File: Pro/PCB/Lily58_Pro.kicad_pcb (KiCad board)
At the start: 2 copper layers, 142.5 x 111.4 mm, 58 parts, among them J1 OLED, J2 TRRS, SW1 SW_PUSH, SW10 SW_PUSH, SW11 SW_PUSH, SW12 SW_PUSH, SW13 SW_PUSH, SW14 SW_PUSH, SW15 SW_PUSH, SW16 SW_PUSH, SW17 SW_PUSH, SW18 SW_PUSH, SW19 SW_PUSH, SW2 SW_PUSH, SW20 SW_PUSH, SW21 SW_PUSH, SW22 SW_PUSH, SW23 SW_PUSH, SW24 SW_PUSH, SW25 SW_PUSH, SW26 SW_PUSH, SW27 SW_PUSH, SW28 SW_PUSH, SW29 SW_PUSH, SW3 SW_PUSH, SW4 SW_PUSH, SW5 SW_PUSH, SW6 SW_PUSH, SW7 SW_PUSH, SW8 SW_PUSH, SW9 SW_PUSH

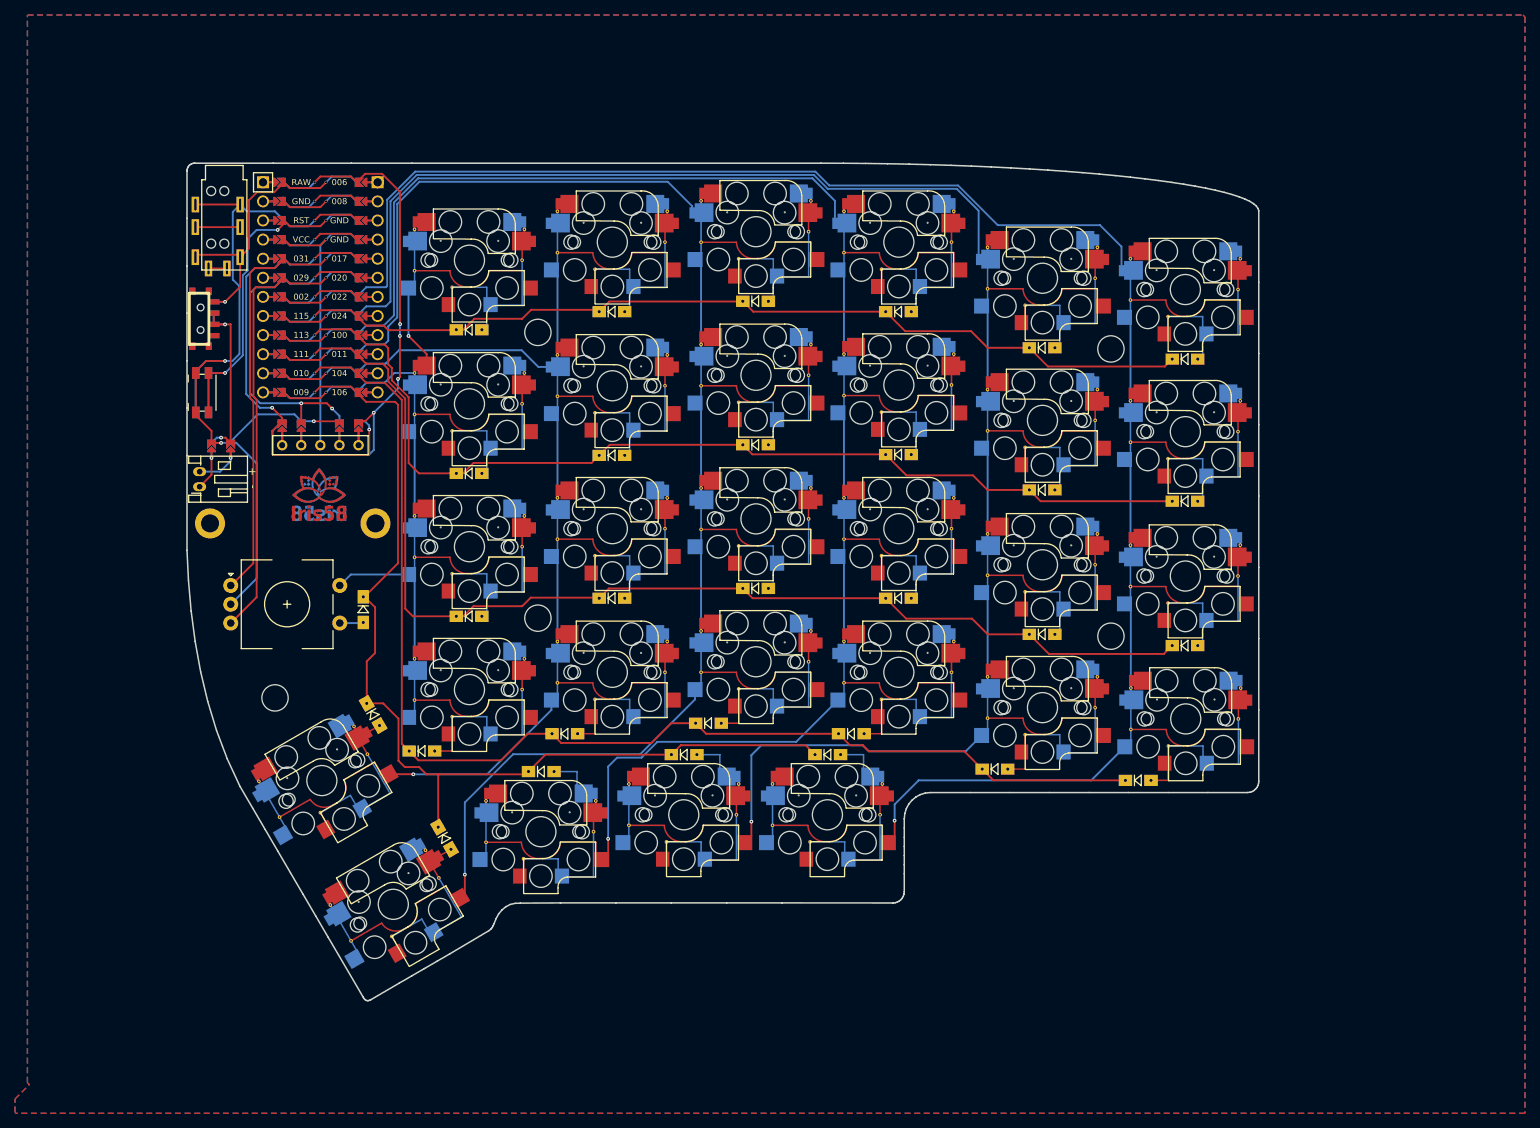
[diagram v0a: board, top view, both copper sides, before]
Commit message: Small fixes
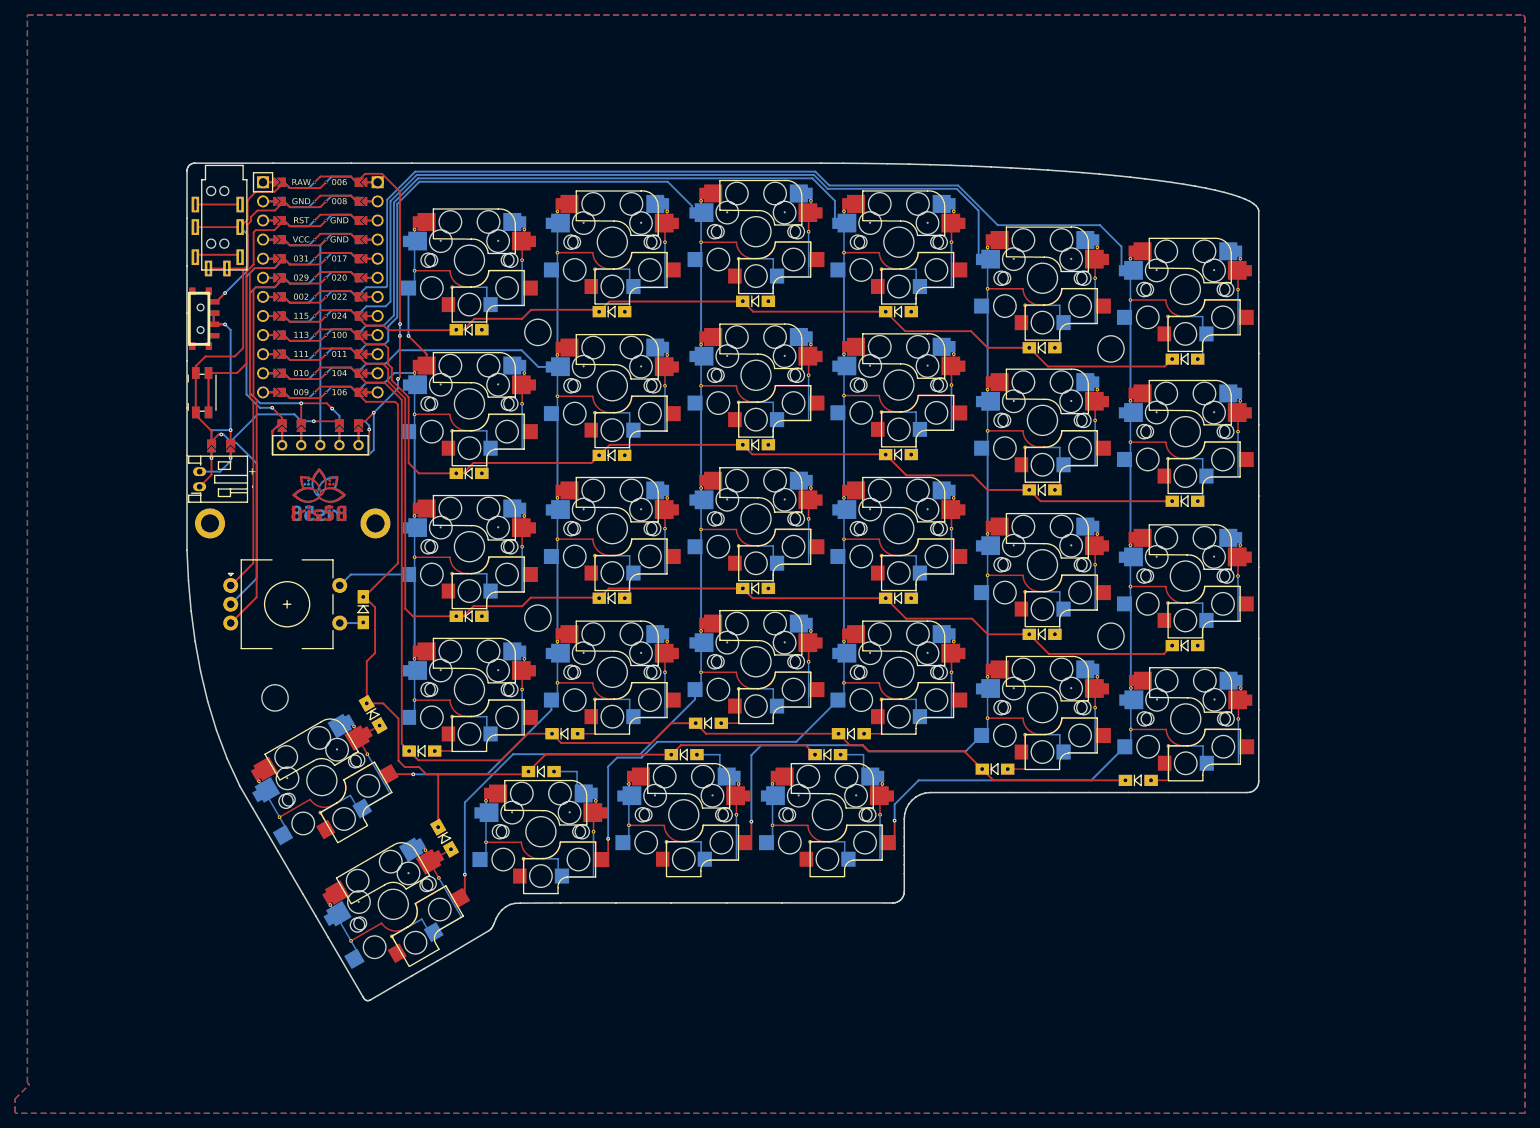
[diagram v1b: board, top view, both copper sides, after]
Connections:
- J2 pad 1: RAW -> unconnected-(J2-Pad1)
- J2 pad 2: unconnected-(J2-Pad2) -> RAW
- J2 pad 3: GND -> unconnected-(J2-Pad3)
- J2 pad 4: unconnected-(J2-Pad4) -> GND
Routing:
- net GND: track 104.1 -> 90.6 mm, vias 3 -> 2
- net unconnected-(J2-Pad3): track 0.00 -> 5.95 mm
- net unconnected-(J2-Pad2): track 5.95 -> 0.00 mm
- net unconnected-(J2-Pad1): track 0.00 -> 5.30 mm
- net unconnected-(J2-Pad4): track 2.45 -> 0.00 mm
- net RESET: track 39.5 -> 38.6 mm, vias 2 -> 0
- net BAT_POS: track 25.5 -> 26.3 mm
- net RAW: track 28.8 -> 29.5 mm
